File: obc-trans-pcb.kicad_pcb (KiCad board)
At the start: 4 copper layers, 95.9 x 90.2 mm, 31 parts, among them IC1 DS3234, J1 H1, J2 H2, J3 H_EPS, J4 DEBUGGING PORT, J5 PROGRAMMING PORT, SW1 SW_RST, U1 SN65HVD230, U2 ATMEGA32M1-MU, U3 SST25VF016B, U4 SST25VF016B, U5 SST25VF016B, Y1 8 MHz

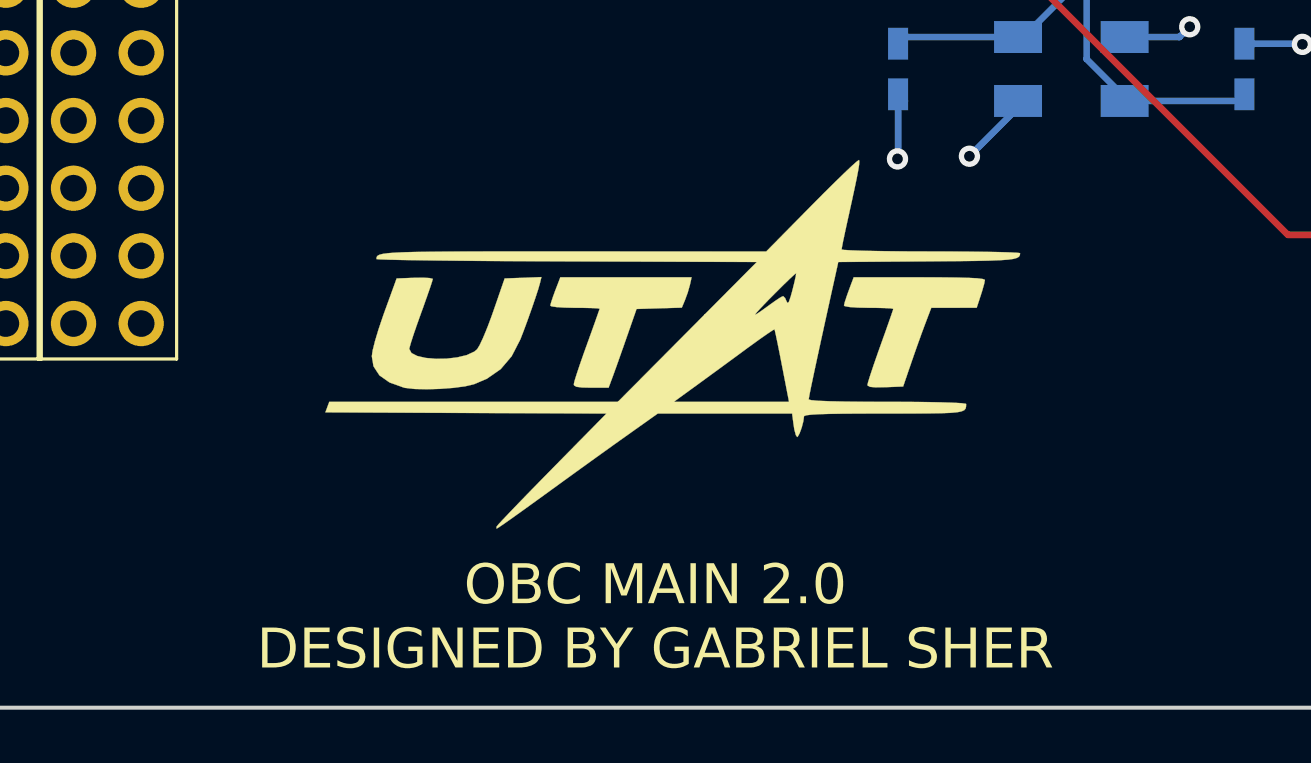
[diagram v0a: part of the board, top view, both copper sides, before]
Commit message: Revert "text added"
This reverts commit e1df546076587439d09c56251eebff1379ce6698.
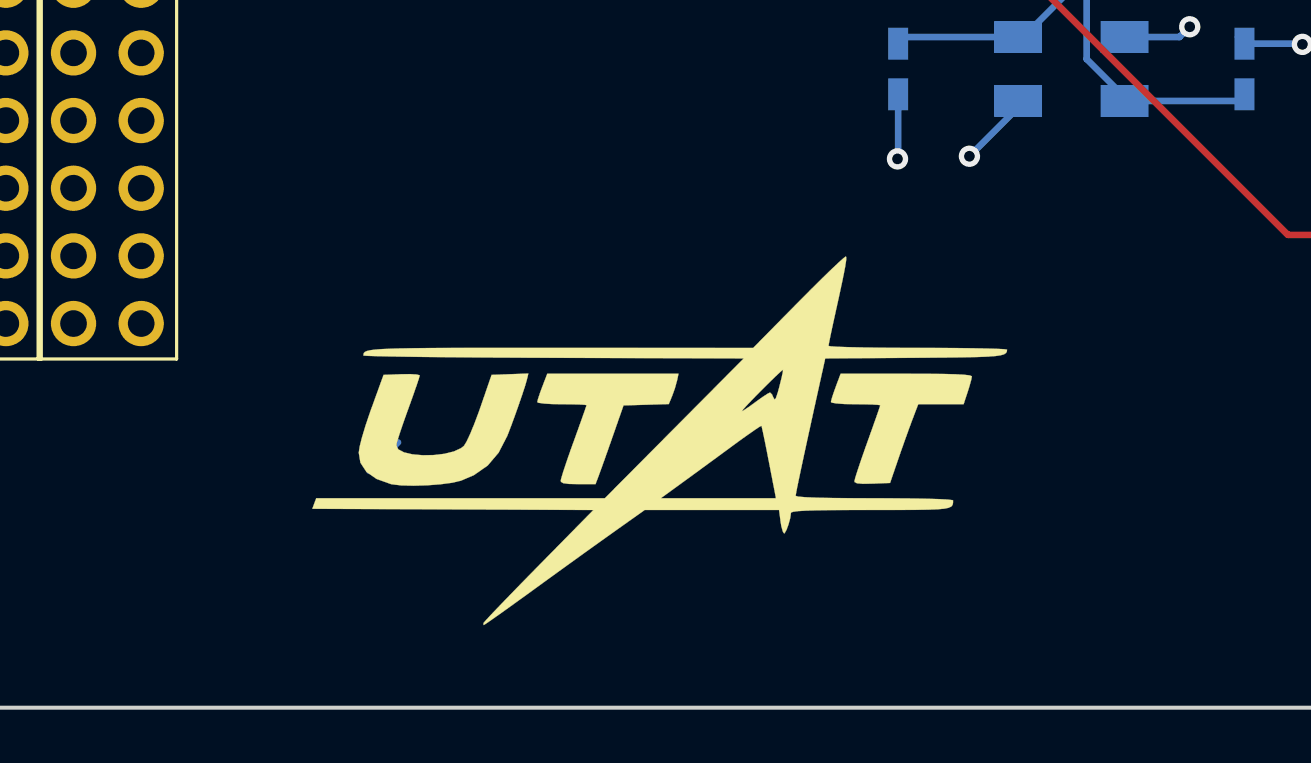
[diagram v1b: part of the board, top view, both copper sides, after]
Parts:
- moved G*** 3.65 mm to (132.8, 129.6)
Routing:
- net GND: track 85.8 -> 87.3 mm, vias 24 -> 28
- net (no net): vias 4 -> 0
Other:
- board text removed: "OBC MAIN 2.0 DESIGNED BY GABRIEL SHER"
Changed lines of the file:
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@@
     (links 117)
     (no_connects 0)
-    (area 99.589999 49.309999 196.520002 140.520002)
+    (area 98.589999 48.309999 197.520002 141.520002)
     (thickness 1.6)
-    (drawings 5)
-    (tracks 477)
+    (drawings 4)
+    (tracks 478)
     (zones 0)
     (modules 31)
@@
   )
   (module obc-trans-pcb:utat-logo (layer F.Cu)
-    (at 133.24 125.96)
+    (at 132.75 129.58)
     (fp_text reference G*** (at 0 0) (layer F.SilkS) hide
       (effects (font (thickness 0.3)))
@@
       (xy 6.532726 -1.628289) (xy 6.715451 -2.116667) (xy 9.178559 -2.116667) (xy 9.956872 -2.114533)) (layer F.SilkS) (width 0.01))
   )
-  (gr_text "OBC MAIN 2.0\nDESIGNED BY GABRIEL SHER" (at 132.51 136.59) (layer F.SilkS)
-    (effects (font (size 1.5 1.5) (thickness 0.3)))
-  )
   (gr_line (start 100.11 140) (end 196 140) (angle 90) (layer Edge.Cuts) (width 0.15))
   (gr_line (start 100.11 49.83) (end 100.11 140) (angle 90) (layer Edge.Cuts) (width 0.15))
   (gr_line (start 196 49.83) (end 100.11 49.83) (angle 90) (layer Edge.Cuts) (width 0.15))
   (gr_line (start 196 49.83) (end 196 140) (angle 90) (layer Edge.Cuts) (width 0.15))
-  (via (at 105.19 131.11) (size 5.4) (drill 3.2) (layers F.Cu B.Cu) (net 0))
-  (via (at 190.92 134.92) (size 5.4) (drill 3.2) (layers F.Cu B.Cu) (net 0))
-  (via (at 190.92 54.91) (size 5.4) (drill 3.2) (layers F.Cu B.Cu) (net 0))
-  (via (at 105.19 57.45) (size 5.4) (drill 3.2) (layers F.Cu B.Cu) (net 0))
+  (via (at 105.19 131.11) (size 5.4) (drill 3.2) (layers F.Cu B.Cu) (net 1))
+  (segment (start 122.85 130.04) (end 121.78 131.11) (width 0.25) (layer B.Cu) (net 1))
+  (via (at 190.92 134.92) (size 5.4) (drill 3.2) (layers F.Cu B.Cu) (net 1))
+  (via (at 190.92 54.91) (size 5.4) (drill 3.2) (layers F.Cu B.Cu) (net 1))
+  (via (at 105.19 57.45) (size 5.4) (drill 3.2) (layers F.Cu B.Cu) (net 1))
   (segment (start 161.805 78.05) (end 161.805 77.005) (width 0.25) (layer B.Cu) (net 1))
   (via (at 160.25 75.45) (size 0.8) (drill 0.4) (layers F.Cu B.Cu) (net 1))

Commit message: text added
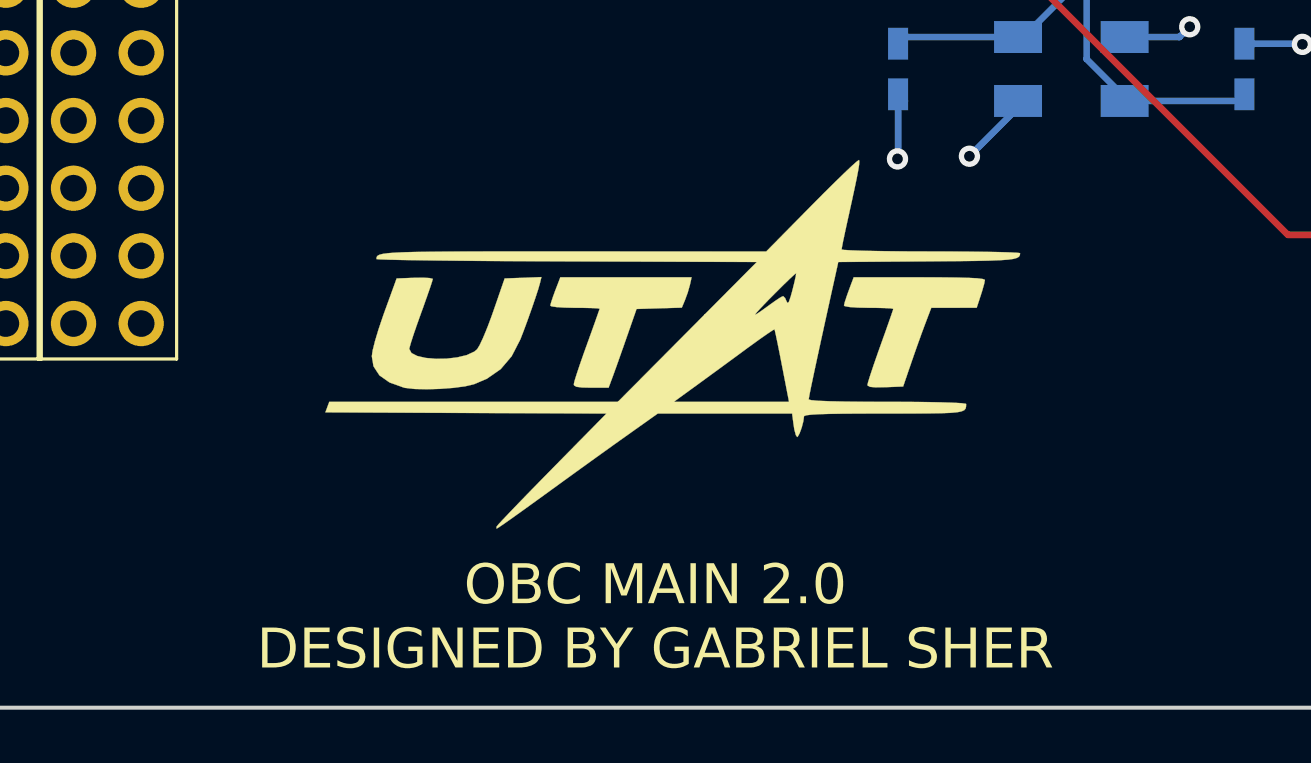
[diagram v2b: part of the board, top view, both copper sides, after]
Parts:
- moved G*** 3.65 mm to (133.2, 126.0)
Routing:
- net GND: track 87.3 -> 85.8 mm, vias 28 -> 24
- net (no net): vias 0 -> 4
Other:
- board text added: "OBC MAIN 2.0 DESIGNED BY GABRIEL SHER"
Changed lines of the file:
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@@
     (links 117)
     (no_connects 0)
-    (area 98.589999 48.309999 197.520002 141.520002)
+    (area 99.589999 49.309999 196.520002 140.520002)
     (thickness 1.6)
-    (drawings 4)
-    (tracks 478)
+    (drawings 5)
+    (tracks 477)
     (zones 0)
     (modules 31)
@@
   )
   (module obc-trans-pcb:utat-logo (layer F.Cu)
-    (at 132.75 129.58)
+    (at 133.24 125.96)
     (fp_text reference G*** (at 0 0) (layer F.SilkS) hide
       (effects (font (thickness 0.3)))
@@
       (xy 6.532726 -1.628289) (xy 6.715451 -2.116667) (xy 9.178559 -2.116667) (xy 9.956872 -2.114533)) (layer F.SilkS) (width 0.01))
   )
+  (gr_text "OBC MAIN 2.0\nDESIGNED BY GABRIEL SHER" (at 132.51 136.59) (layer F.SilkS)
+    (effects (font (size 1.5 1.5) (thickness 0.3)))
+  )
   (gr_line (start 100.11 140) (end 196 140) (angle 90) (layer Edge.Cuts) (width 0.15))
   (gr_line (start 100.11 49.83) (end 100.11 140) (angle 90) (layer Edge.Cuts) (width 0.15))
   (gr_line (start 196 49.83) (end 100.11 49.83) (angle 90) (layer Edge.Cuts) (width 0.15))
   (gr_line (start 196 49.83) (end 196 140) (angle 90) (layer Edge.Cuts) (width 0.15))
-  (via (at 105.19 131.11) (size 5.4) (drill 3.2) (layers F.Cu B.Cu) (net 1))
-  (segment (start 122.85 130.04) (end 121.78 131.11) (width 0.25) (layer B.Cu) (net 1))
-  (via (at 190.92 134.92) (size 5.4) (drill 3.2) (layers F.Cu B.Cu) (net 1))
-  (via (at 190.92 54.91) (size 5.4) (drill 3.2) (layers F.Cu B.Cu) (net 1))
-  (via (at 105.19 57.45) (size 5.4) (drill 3.2) (layers F.Cu B.Cu) (net 1))
+  (via (at 105.19 131.11) (size 5.4) (drill 3.2) (layers F.Cu B.Cu) (net 0))
+  (via (at 190.92 134.92) (size 5.4) (drill 3.2) (layers F.Cu B.Cu) (net 0))
+  (via (at 190.92 54.91) (size 5.4) (drill 3.2) (layers F.Cu B.Cu) (net 0))
+  (via (at 105.19 57.45) (size 5.4) (drill 3.2) (layers F.Cu B.Cu) (net 0))
   (segment (start 161.805 78.05) (end 161.805 77.005) (width 0.25) (layer B.Cu) (net 1))
   (via (at 160.25 75.45) (size 0.8) (drill 0.4) (layers F.Cu B.Cu) (net 1))
